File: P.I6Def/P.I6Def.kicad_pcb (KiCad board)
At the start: 2 copper layers, 45.8 x 59.2 mm, 41 parts, among them J1 B3B-PH-K-S, J2 B3B-PH-K-S, J3 CX90B-16P1, J4 B4B-PH-SM4-TB_LF__SN__P_, J5 B4B-PH-SM4-TB_LF__SN__P_, SW2 SW_SPST, SW3 SW_SPST, U2 LMV321IDCKT, U3 LMV321IDCKT, U4 LMV321IDCKT, U5 LMV321IDCKT, U6 ESP32-S3-WROOM-1

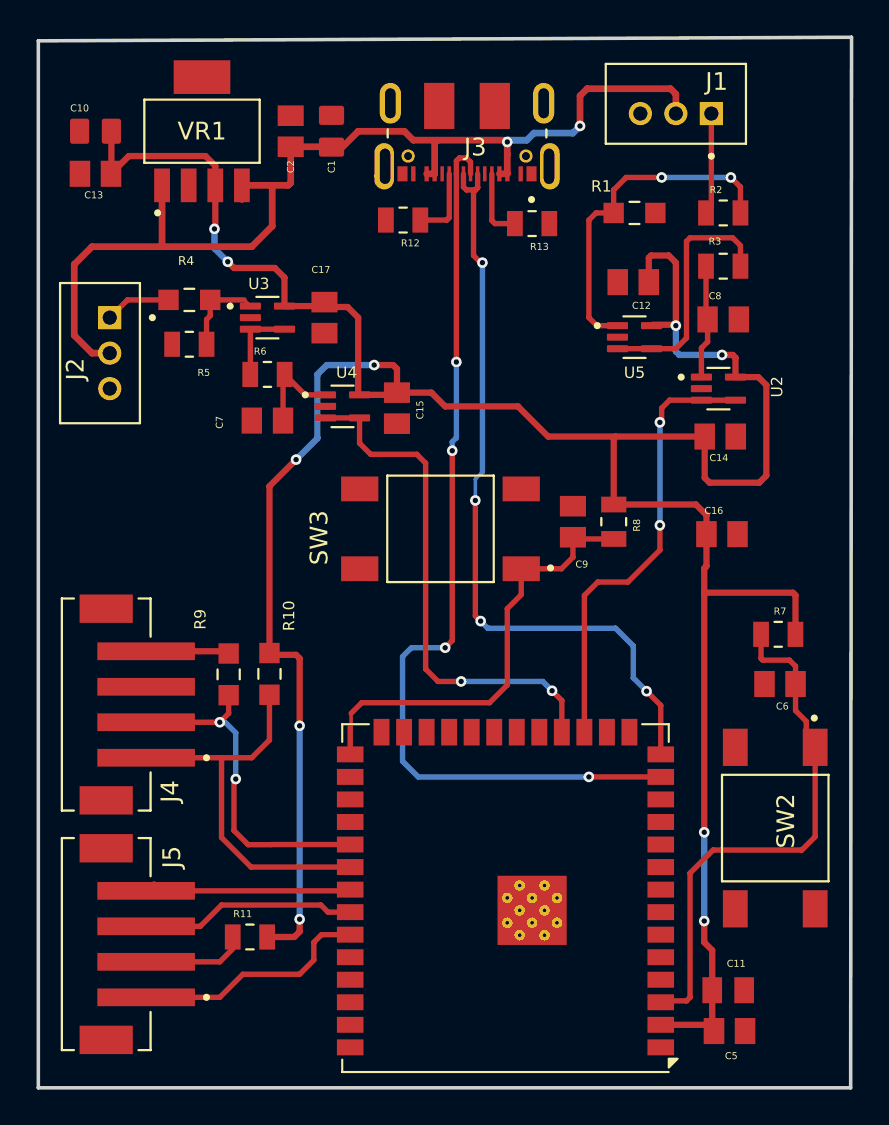
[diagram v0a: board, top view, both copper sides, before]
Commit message: Actualizacion PCB
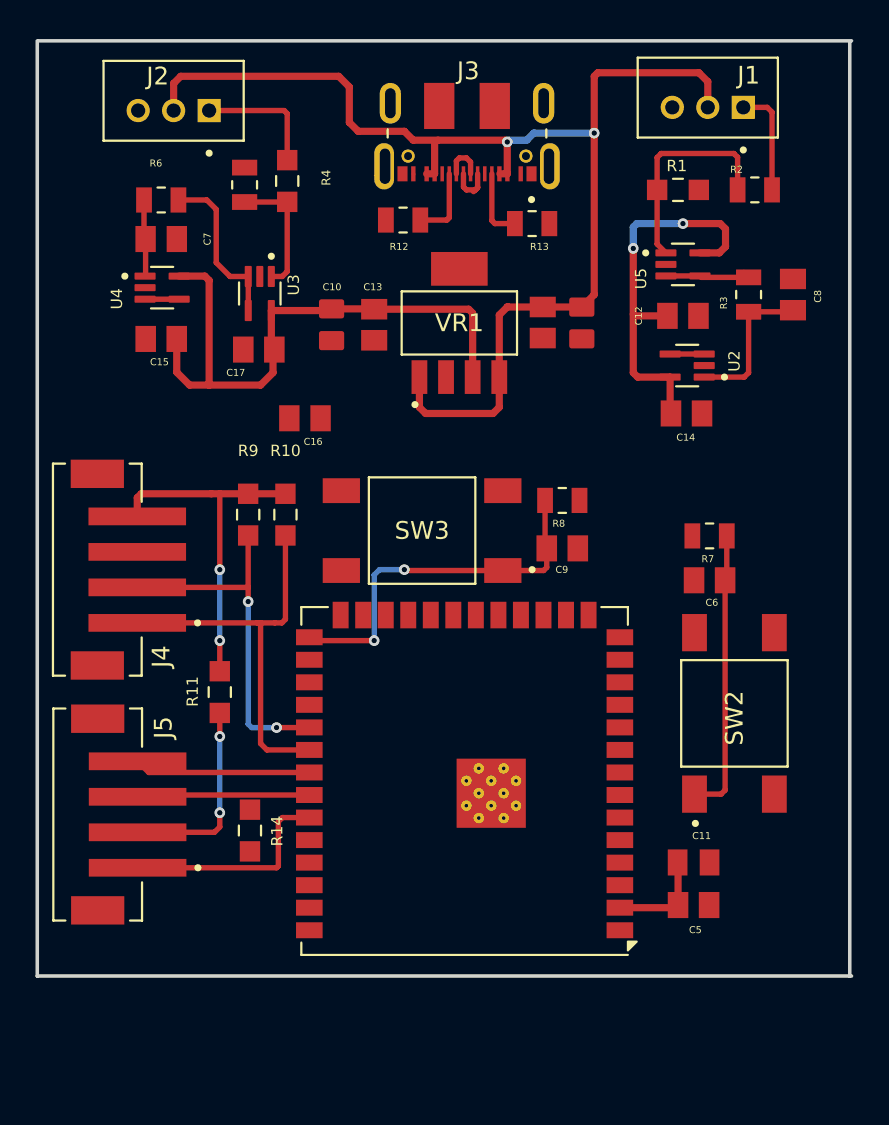
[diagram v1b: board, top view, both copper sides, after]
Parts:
- added R14: 4.7k, ERA6AEB472V:RES_ERA6AEB472V, F.Cu at (112.4, 89.4)
- C16: value 0.1u -> 1uF; footprint C0805C104K8RACTU:CAPC2012X88N -> C2012X5R1C105K085AA:CAPC2012X100N
- R11: value 10k -> 4.7k; footprint MCU08050C1002FP500:RESC2012X55N -> ERA6AEB472V:RES_ERA6AEB472V
- moved C16 24.4 mm to (115.5, 66.2), turned to 180 degrees
- moved VR1 18.1 mm to (124.2, 60.8)
- moved C13 17.9 mm to (119.4, 60.9), turned to -90 degrees
- moved C2 17.8 mm to (128.9, 60.8), turned to -90 degrees
- moved C1 17.8 mm to (131.1, 60.8), turned to -90 degrees
- moved C10 17.2 mm to (117.0, 60.9), turned to -90 degrees
- moved J2 14.8 mm to (108.1, 48.3), turned to 0 degrees
- moved R11 13.9 mm to (110.7, 81.6), turned to 90 degrees
- moved C15 13.8 mm to (107.4, 61.7), turned to 180 degrees
- moved U4 12.2 mm to (107.5, 58.8)
- moved C7 11.9 mm to (107.4, 56.1), turned to 0 degrees
- moved R6 11.5 mm to (107.4, 53.9), turned to 180 degrees
- moved R5 9.51 mm to (112.1, 53.0), turned to -90 degrees
- moved R9 9.07 mm to (112.3, 71.6)
- moved R10 9.02 mm to (114.4, 71.6)
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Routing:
- net +3.3V: track 172.9 -> 82.4 mm, vias 10 -> 4
- net /D-: track 52.7 -> 2.36 mm, vias 4 -> 0
- net /D+: track 43.4 -> 2.76 mm, vias 4 -> 0
- net /ADC1_CH1: track 29.3 -> 1.92 mm, vias 2 -> 0
- net /ADC1_CH0: track 25.5 -> 1.92 mm, vias 2 -> 0
- net Net-(SW2-A): track 30.2 -> 16.2 mm
- net +5V: track 60.5 -> 70.7 mm
- net Net-(U5-1IN-): track 14.1 -> 5.09 mm
- net Net-(U5-1IN+): track 19.3 -> 12.1 mm, vias 2 -> 0
- net Net-(J5-Pad2): track 5.85 -> 11.4 mm, vias 0 -> 2
- net Net-(U3-1IN-): track 4.47 -> 9.40 mm
- net /BOOT: track 25.3 -> 21.2 mm, vias 0 -> 2
- net Net-(J2-Pad1): track 3.72 -> 7.10 mm
- net /nINT_CCS811: track 12.2 -> 9.72 mm
- net Net-(U3-1IN+): track 4.99 -> 7.34 mm
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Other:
- board size 45.8 x 59.2 mm -> 45.9 x 52.7 mm
